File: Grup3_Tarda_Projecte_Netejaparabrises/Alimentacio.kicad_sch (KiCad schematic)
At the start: 8 parts, among them J1 Screw_Terminal_01x02, U1 LM1117MP-5.0

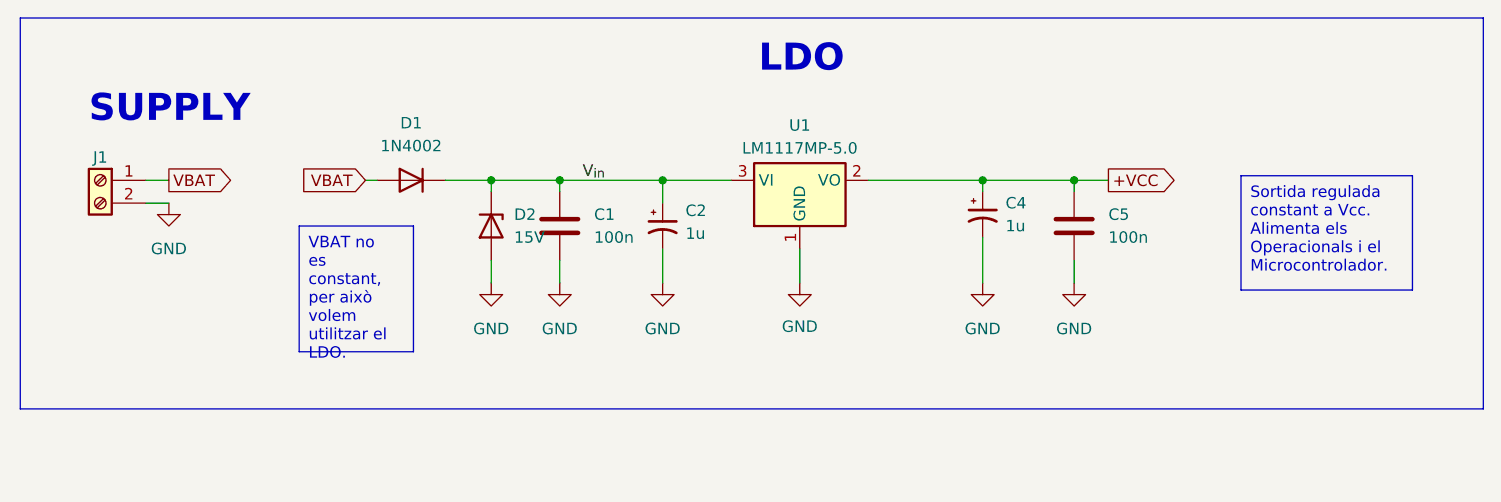
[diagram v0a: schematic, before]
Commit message: canvis schematic 05-04-23
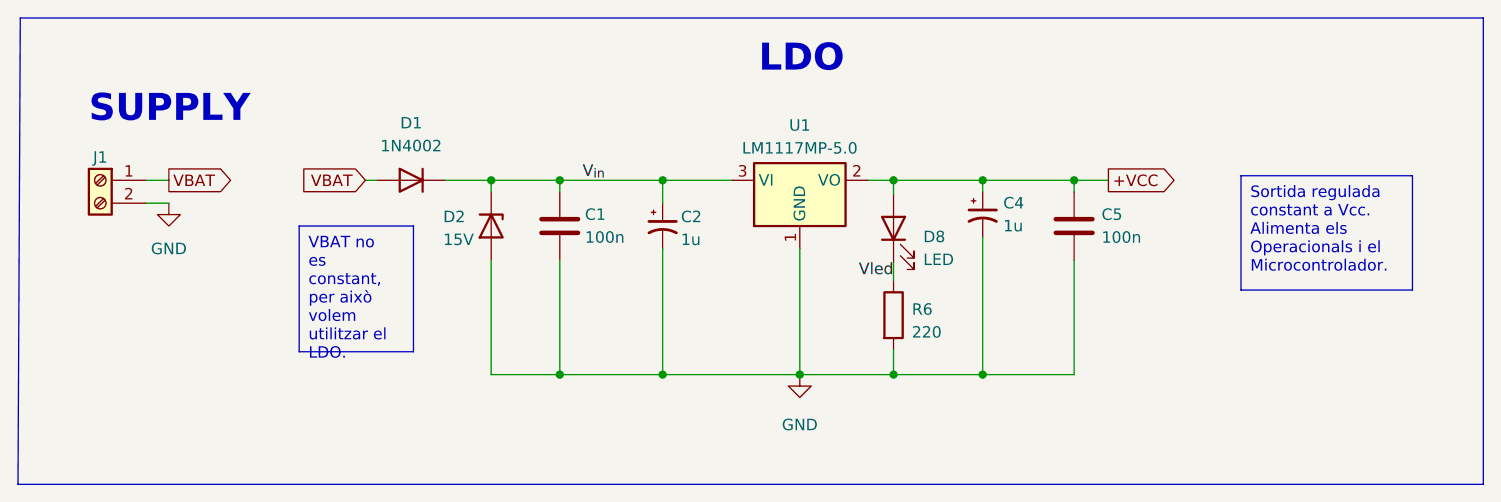
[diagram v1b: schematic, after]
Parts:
- added D8: LED, symbol Device:LED
- added R6: 220, symbol Device:R
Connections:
- net +VCC: now also D8.2 (A)
- net GND: now also R6.2
- new net Vled: D8.1 (K), R6.1
